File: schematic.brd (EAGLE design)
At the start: 32.7 x 24.1 mm, 2 parts, among them J1 USB_A_SMT_FEMALE

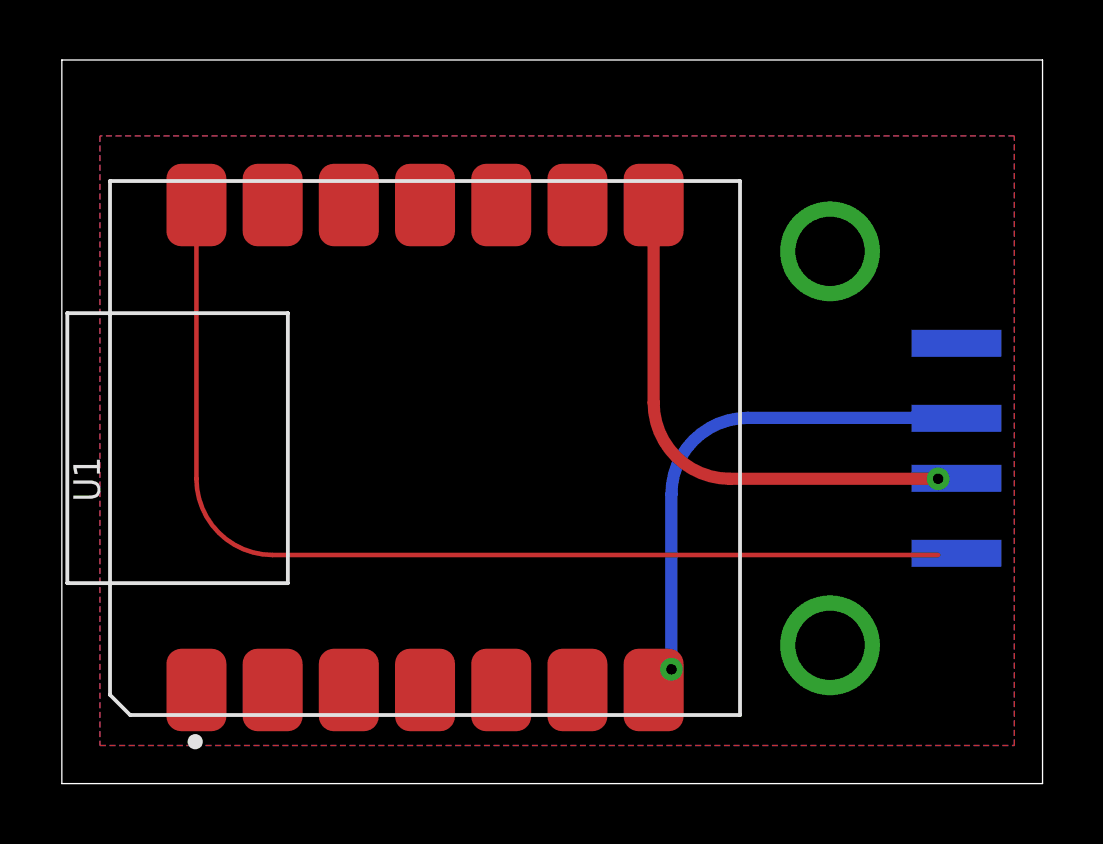
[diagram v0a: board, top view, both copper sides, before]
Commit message: updated schematic and board
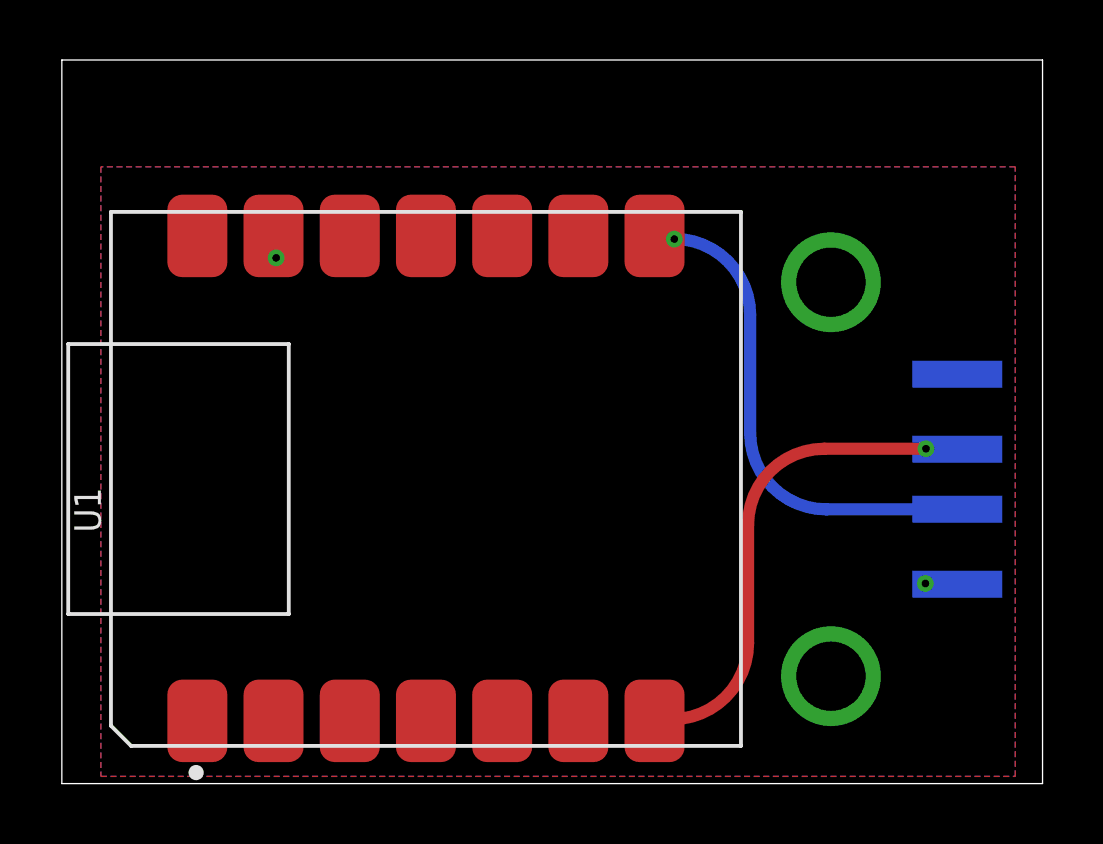
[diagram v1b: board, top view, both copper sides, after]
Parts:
- moved U1 1.03 mm to (22.6, 1.26)
- moved J1 1.03 mm to (22.6, 10.1)
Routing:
- net VCC: track 34.9 -> 1.07 mm, vias 0 -> 1
- net DATA_P: track 0.00 -> 16.3 mm, vias 0 -> 1
- net N$1: track 15.9 -> 0.00 mm, vias 1 -> 0
- net GND: track 0.00 -> 0.76 mm, vias 0 -> 1
- net DATA_N: track 17.1 -> 16.4 mm
- added copper zone on layer 1, net VCC
- removed copper zone on layer 1, net GND
